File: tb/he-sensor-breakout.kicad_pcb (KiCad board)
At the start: 2 copper layers, 19.1 x 17.8 mm, 28 parts, among them J1 Conn_01x01_Pin, J10 Conn_01x01_Pin, J11 Conn_01x01_Pin, J12 Conn_01x01_Pin, J13 Conn_01x01_Pin, J14 Conn_01x01_Pin, J2 Conn_01x01_Pin, J3 Conn_01x01_Pin, J4 Conn_01x01_Pin, J5 Conn_01x01_Pin, J6 Conn_01x01_Pin, J7 Conn_01x01_Pin, J8 Conn_01x01_Pin, J9 Conn_01x01_Pin, U1 SLSS49E

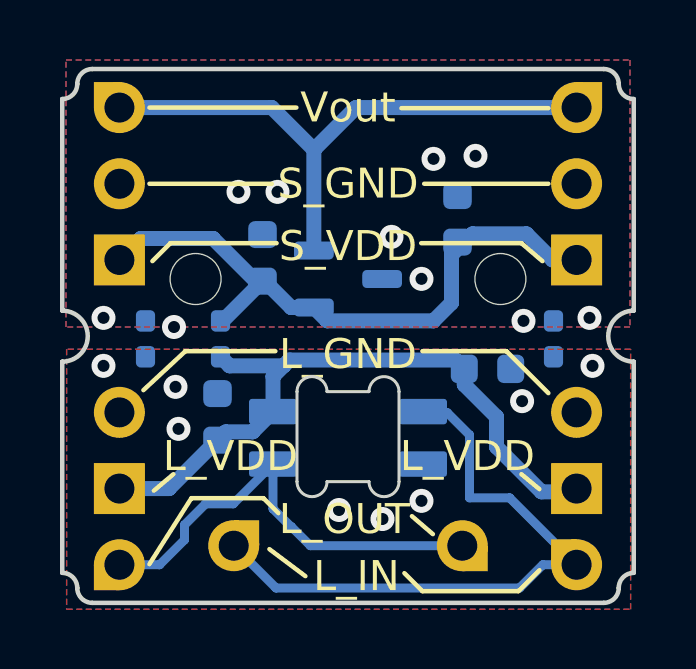
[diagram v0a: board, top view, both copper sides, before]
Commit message: make symmetric
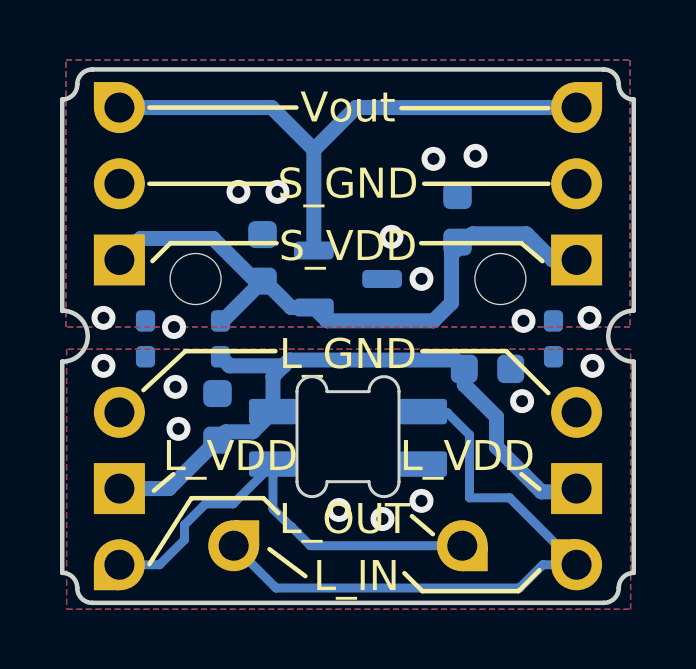
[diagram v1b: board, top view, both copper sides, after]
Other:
- outline, holes or cut-outs redrawn
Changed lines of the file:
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@@
   (gr_arc (start 118.745026 103.6) (mid 116.745 101.6) (end 118.745026 99.6)
     (stroke (width 0.15) (type default)) (layer "Dwgs.User"))
-  (gr_arc (start 100.195 93.195) (mid 100.048553 93.548553) (end 99.695 93.695)
+  (gr_arc (start 100.195 93.21) (mid 100.048553 93.563553) (end 99.695 93.71)
     (stroke (width 0.15) (type default)) (layer "Edge.Cuts"))
   (gr_arc (start 118.745 102.45) (mid 117.895 101.6) (end 118.745 100.75)
     (stroke (width 0.15) (type default)) (layer "Edge.Cuts"))
-  (gr_line (start 99.695 93.695) (end 99.695 100.75)
+  (gr_line (start 99.695 93.71) (end 99.695 100.765)
     (stroke (width 0.15) (type default)) (layer "Edge.Cuts"))
   (gr_line (start 117.745 110.49) (end 100.695 110.49)
@@
   (gr_line (start 118.745 102.45) (end 118.745 109.49)
     (stroke (width 0.15) (type default)) (layer "Edge.Cuts"))
-  (gr_line (start 118.745 93.695) (end 118.745 100.75)
+  (gr_line (start 118.745 93.71) (end 118.745 100.75)
     (stroke (width 0.15) (type default)) (layer "Edge.Cuts"))
   (gr_line (start 99.695 102.45) (end 99.695 109.49)
@@
   (gr_arc (start 99.695 100.75) (mid 100.545 101.6) (end 99.695 102.45)
     (stroke (width 0.15) (type default)) (layer "Edge.Cuts"))
-  (gr_line (start 100.695 92.695) (end 117.745 92.695)
+  (gr_line (start 100.695 92.71) (end 117.745 92.71)
     (stroke (width 0.15) (type default)) (layer "Edge.Cuts"))
-  (gr_arc (start 100.195 93.195) (mid 100.341447 92.841447) (end 100.695 92.695)
+  (gr_arc (start 100.195 93.21) (mid 100.341447 92.856447) (end 100.695 92.71)
     (stroke (width 0.15) (type default)) (layer "Edge.Cuts"))
   (gr_arc (start 118.245 109.99) (mid 118.098612 110.343612) (end 117.745 110.49)
     (stroke (width 0.15) (type default)) (layer "Edge.Cuts"))
-  (gr_arc (start 117.745 92.695) (mid 118.098553 92.841447) (end 118.245 93.195)
+  (gr_arc (start 117.745 92.71) (mid 118.098553 92.856447) (end 118.245 93.21)
     (stroke (width 0.15) (type default)) (layer "Edge.Cuts"))
   (gr_arc (start 99.695 109.49) (mid 100.048553 109.636447) (end 100.195 109.99)
     (stroke (width 0.15) (type default)) (layer "Edge.Cuts"))
-  (gr_arc (start 118.745 93.695) (mid 118.391447 93.548553) (end 118.245 93.195)
+  (gr_arc (start 118.745 93.71) (mid 118.391447 93.563553) (end 118.245 93.21)
     (stroke (width 0.15) (type default)) (layer "Edge.Cuts"))
   (gr_arc (start 100.695 110.49) (mid 100.341447 110.343553) (end 100.195 109.99)
